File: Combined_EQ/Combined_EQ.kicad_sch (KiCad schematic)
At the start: 25 parts, among them IC2 OPA1644AIPWR

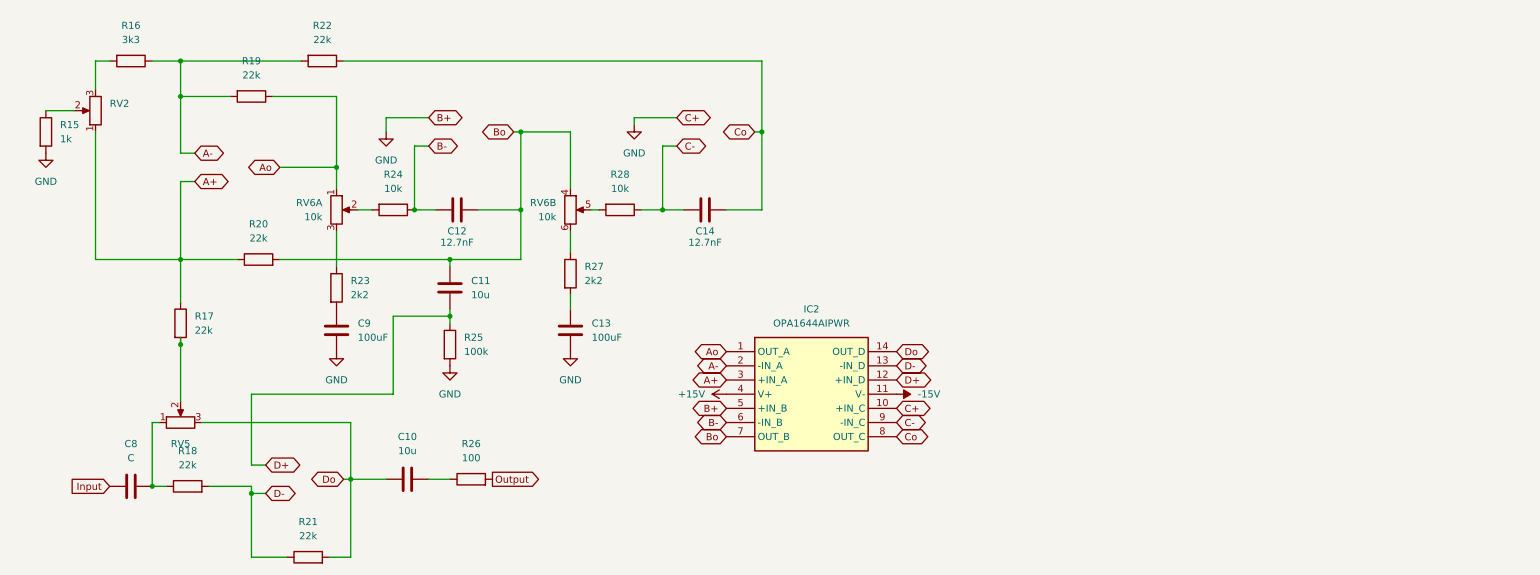
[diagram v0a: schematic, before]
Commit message: yurrrr
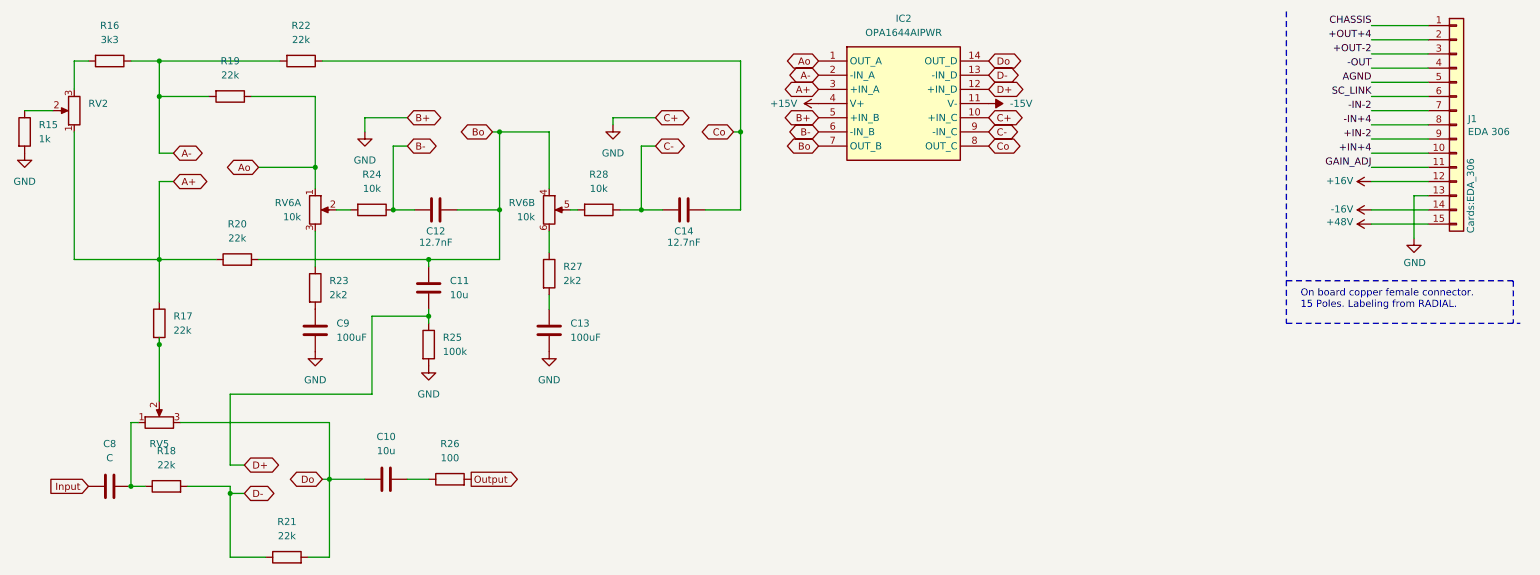
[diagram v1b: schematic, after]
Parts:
- added J1: EDA 306, Cards:EDA_306, symbol Connector_Generic:Conn_01x15
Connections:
- net GND: now also J1.13 (Pin_13)
- new net +16V: J1.12 (Pin_12)
- new net +48V: J1.15 (Pin_15)
- new net +IN+4: J1.10 (Pin_10)
- new net +IN-2: J1.9 (Pin_9)
- new net +OUT+4: J1.2 (Pin_2)
- new net +OUT-2: J1.3 (Pin_3)
- new net -16V: J1.14 (Pin_14)
- new net -IN+4: J1.8 (Pin_8)
- new net -IN-2: J1.7 (Pin_7)
- new net -OUT: J1.4 (Pin_4)
- new net AGND: J1.5 (Pin_5)
- new net CHASSIS: J1.1 (Pin_1)
- new net GAIN_ADJ: J1.11 (Pin_11)
- new net SC_LINK: J1.6 (Pin_6)
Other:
- note added: "On board copper female connector. 15 Poles. Labeling from RADIAL."
- title: High Bandpass Filter -> API Series 500 (EDA 306)
- moved on the sheet: C10, C11, C12, C13, C14, C8, C9, IC2, R15, R16, R17, R18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

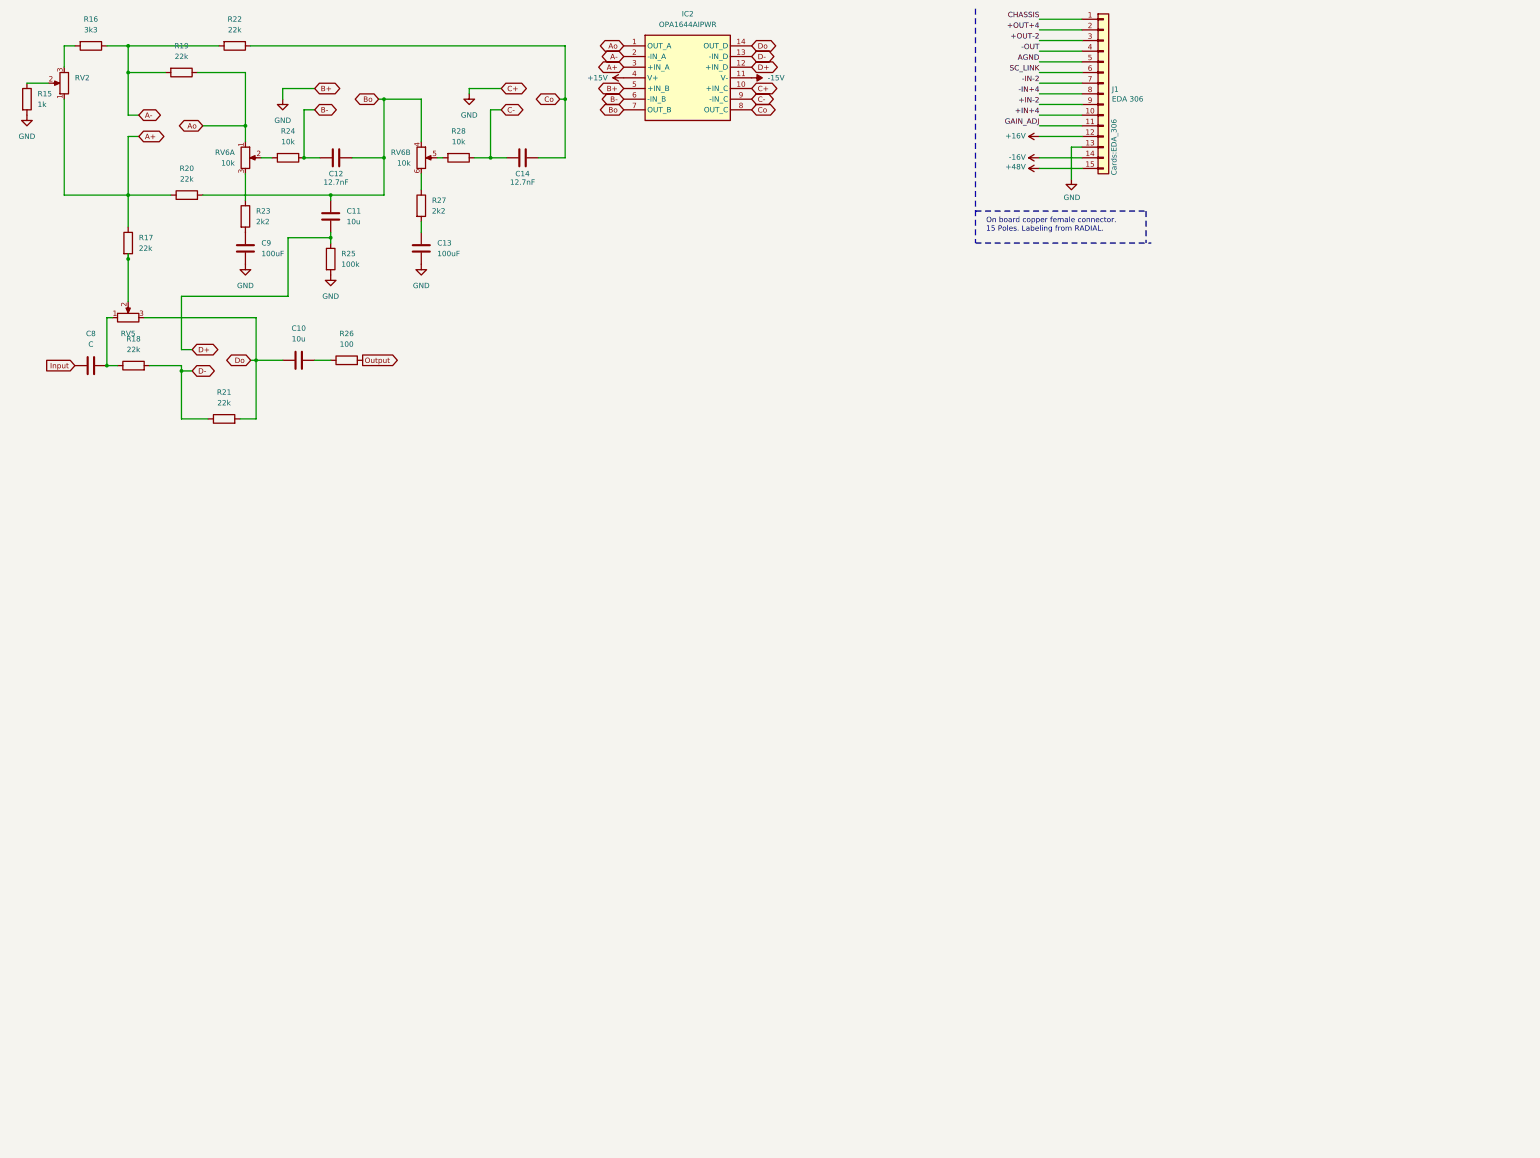
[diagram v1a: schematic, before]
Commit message: started main schematic
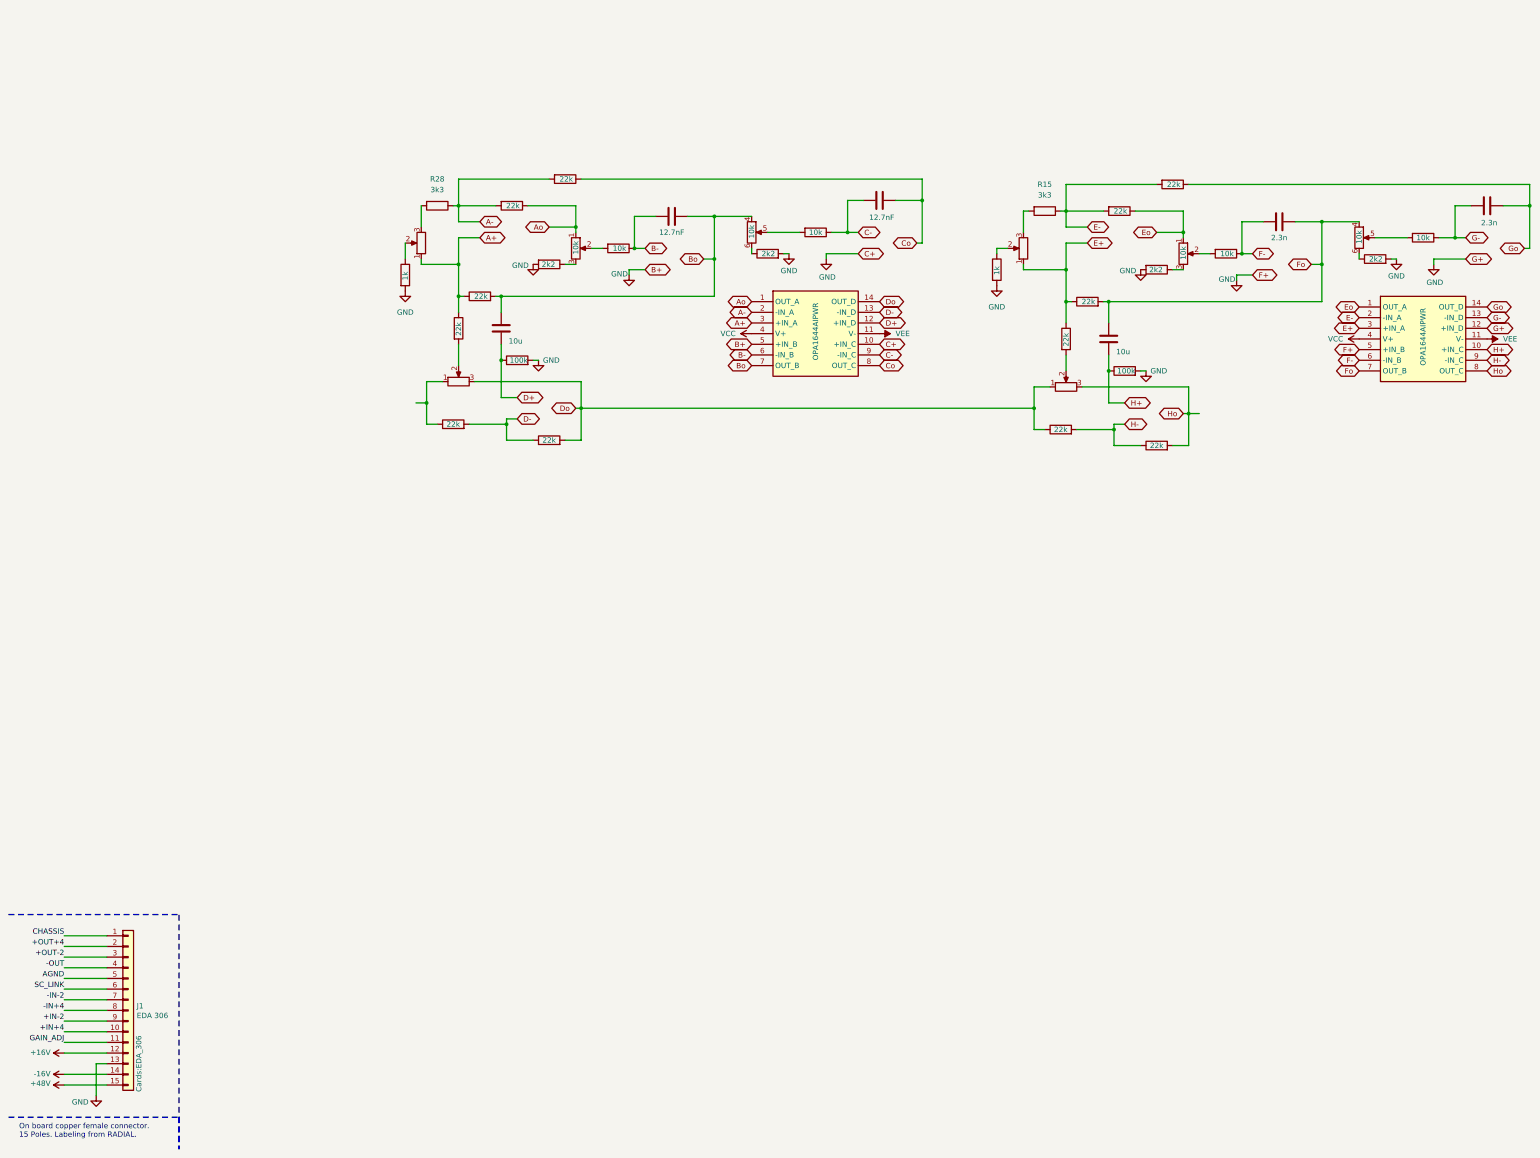
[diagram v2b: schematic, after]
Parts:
- removed C10, C11: 10u, symbol Device:C
- removed C12, C14: 12.7nF, symbol Device:C
- removed C13: 100uF, symbol Device:C
- added C2, C7: 10u, symbol Device:C
- added C3, C6: 2.3n, symbol Device:C
- added IC3: OPA1644AIPWR, SOP65P640X120-14N, symbol OPA1644AIPWR:OPA1644AIPWR
- added R14: 1k, Resistor_THT:R_Axial_DIN0207_L6.3mm_D2.5mm_P10.16mm_Horizontal, symbol Device:R
- added R29, R30, R31, R32, R35, R39: 22k, Resistor_THT:R_Axial_DIN0207_L6.3mm_D2.5mm_P10.16mm_Horizontal, symbol Device:R
- added R33: 100k, Resistor_THT:R_Axial_DIN0207_L6.3mm_D2.5mm_P10.16mm_Horizontal, symbol Device:R
- added R34, R37: 2k2, Resistor_THT:R_Axial_DIN0207_L6.3mm_D2.5mm_P10.16mm_Horizontal, symbol Device:R
- added R36, R38: 10k, Resistor_THT:R_Axial_DIN0207_L6.3mm_D2.5mm_P10.16mm_Horizontal, symbol Device:R
- added RV7, RV8: 10k, symbol Device:R_Potentiometer
- added RV9: 10k, symbol Device:R_Potentiometer_Dual_Separate
- C8: value C -> 12.7nF
- C9: value 100uF -> 12.7nF
- R15: value 1k -> 3k3
- R16: value 3k3 -> 22k
- R20: value 22k -> 100k
- R21: value 22k -> 2k2
- R23: value 2k2 -> 22k
- R25: value 100k -> 2k2
- R26: value 100 -> 10k
- R27: value 2k2 -> 1k
- R28: value 10k -> 3k3
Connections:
- net Input is gone; now on net Bo: C8.2
- net Output is gone; now on an unnamed net: R26.2
- net A+: now also IC3.3 (+IN_A), R30.1, R31.1, RV7.1; no longer IC2.3 (+IN_A), R17.1, R20.1, RV2.1
- net A-: now also R28.1, IC3.2 (-IN_A), R32.2, R35.2; no longer IC2.2 (-IN_A), R16.1, R19.2, R22.2
- net Ao: now also IC3.1 (OUT_A), R32.1, RV9.1; no longer IC2.1 (OUT_A), R19.1, RV6.1
- net B-: now also C8.1, IC3.6 (-IN_B), R36.1; no longer IC2.6 (-IN_B), R24.1
- net Bo: now also C7.2, IC3.7 (OUT_B), R31.2, RV9.4; no longer IC2.7 (OUT_B), R20.2, RV6.4
- net C-: now also C9.1, IC3.9 (-IN_C), R38.1; no longer IC2.9 (-IN_C), R28.1
- net Co: now also C9.2, IC3.8 (OUT_C), R35.1; no longer IC2.8 (OUT_C), R22.1
- net D+: now also C7.1, IC3.12 (+IN_D), R33.1; no longer IC2.12 (+IN_D), R25.1
- net D-: now also IC3.13 (-IN_D), R29.2, R39.1; no longer IC2.13 (-IN_D), R18.2, R21.1
- net Do: now also R16.1, RV5.1, IC3.14 (OUT_D), R39.2, RV8.3; no longer IC2.14 (OUT_D), R21.2, RV5.3
- net GND: now also IC2.12 (+IN_D), R20.2, R21.2, R27.2, IC3.10 (+IN_C), IC3.5 (+IN_B), R14.2, R33.2, R34.2, R37.2; no longer C9.1, IC2.10 (+IN_C), R15.2
- net at RV2.3: now also R15.2; no longer R16.2
- net at RV2.2: now also R14.1; no longer R15.1
- net at RV6.3: now also R21.1; no longer R23.1
- net E-: now reaches R23.2
- net E-: now also IC2.2 (-IN_A), R15.1, R19.2; no longer C9.2
- net G-: now reaches R26.1
- net G-: now also IC2.13 (-IN_D), C6.1
- net at RV6.5: no longer R28.2
- net at R27.1: now also RV7.2; no longer RV6.6
- net +15V renamed VCC
- net VCC: now also IC3.4 (V+)
- net -15V renamed VEE
- net VEE: now also IC3.11 (V-)
- new net: R38.2, RV9.5
- new net: R29.1, RV8.1
- new net: R30.2, RV8.2
- new net: R37.1, RV9.6
- new net: R28.2, RV7.3
- new net: R34.1, RV9.3
- new net: R25.1, RV6.6
- new net: R36.2, RV9.2
- new net E+: IC2.3 (+IN_A), R17.1, R18.1, RV2.1
- new net Eo: IC2.1 (OUT_A), R19.1, RV6.1
- new net F-: C3.1, IC2.6 (-IN_B), R24.1
- new net Fo: C2.2, C3.2, IC2.7 (OUT_B), R18.2, RV6.4
- new net Go: C6.2, IC2.14 (OUT_D), R23.1
- new net H+: C2.1, IC2.10 (+IN_C), R20.1
- new net H-: IC2.9 (-IN_C), R16.2, R22.1
- new net Ho: IC2.8 (OUT_C), R22.2, RV5.3
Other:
- moved on the sheet: J1

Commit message: worked on combined eq plus fixed a few things in gain, LPF and Bandpass
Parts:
- added C1, C5: 470p, symbol Device:C
- added C10, C4: 47u, symbol Device:C
- added C11, C12, C23: 1u, symbol Device:C
- added C13, C14, C15, C16, C17, C19, C21, C22, C30, C31: 100n, symbol Device:C
- added C18, C20, C28, C32: 100u, symbol Device:C
- added C24, C27: 20n, symbol Device:C
- added C25, C26: 270p, symbol Device:C
- added C29, C33: 220p, symbol Device:C
- added IC1: INA137PA, DIP794W53P254L959H508Q8N, symbol INA137PA:INA137PA
- added IC4, IC5: OPA1644AIPWR, OPA1644:SOP65P640X120-14N, symbol OPA1644AIPWR:OPA1644AIPWR
- added R1, R3: 47, symbol Device:R
- added R10, R41: 27K, symbol Device:R
- added R11, R43: 16K, symbol Device:R
- added R12: 5.6K, symbol Device:R
- added R13, R44: 10K, symbol Device:R
- added R2, R4, R7: 100k, symbol Device:R
- added R40, R42: 30K, symbol Device:R
- added R45, R46, R47, R48: 4.7K, symbol Device:R
- added R5, R6: 10, symbol Device:R
- added R8, R9: 6.2K, symbol Device:R
- added RV1, RV4: 100K, symbol Device:R_Potentiometer_Dual_Separate
- added RV10, RV3: 10K, symbol Device:R_Potentiometer
- IC2, IC3: footprint SOP65P640X120-14N -> OPA1644:SOP65P640X120-14N
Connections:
- net AGND is gone; now on net GND: J1.5 (Pin_5)
- net +16V: now also IC3.4 (V+), C12.2, C13.1, C19.2, C20.2, IC1.7 (V+), R6.1; no longer J1.12 (Pin_12)
- net +IN+4: now also R3.1
- net -16V: now also IC2.11 (V-), IC2.4 (V+), IC3.11 (V-), C11.2, C14.1, C15.1, C16.1, C17.1, C18.1, C21.1, C22.1, C30.1, C31.1, IC1.4 (V-), IC4.11 (V-), IC4.4 (V+), IC5.11 (V-), IC5.4 (V+), R5.1; no longer J1.14 (Pin_14)
- net -IN+4: now also R1.1
- net CHASSIS: now also C1.2, C5.2
- net GND: now also C11.1, C12.1, C13.2, C14.2, C15.2, C16.2, C17.2, C18.2, C19.1, C20.1, C21.2, C22.2, C27.1, C30.2, C31.2, IC1.1 (REF), R10.2, R13.2, R2.1, R4.1, R41.2, R7.1, RV4.3
- net Ho: now also C23.1
- net VCC: now also J1.12 (Pin_12), R6.2; no longer IC2.4 (V+), IC3.4 (V+)
- net VEE: now also J1.14 (Pin_14), R5.2; no longer IC2.11 (V-), IC3.11 (V-)
- net I-: now reaches R29.1, RV8.1
- net I-: now also IC4.1 (OUT_A), IC4.2 (-IN_A)
- net +48V: no longer names the net of J1.15 (Pin_15)
- net +IN-2: no longer names the net of J1.9 (Pin_9)
- net +OUT-2: no longer names the net of J1.3 (Pin_3)
- net -IN-2: no longer names the net of J1.7 (Pin_7)
- net GAIN_ADJ: no longer names the net of J1.11 (Pin_11)
- new net: C10.1, C5.1, R3.2
- new net: C10.2, IC1.3 (+IN), R4.2
- new net: C28.1, R45.1
- new net: R8.2, RV1.1, RV1.2
- new net: C4.2, IC1.2 (-IN), R2.2
- new net: C24.2, R9.1, RV1.3
- new net: R9.2, RV1.4, RV1.5
- new net: R48.1, RV10.1
- new net: R47.2, RV10.3
- new net: C1.1, C4.1, R1.2
- new net: C25.2, C26.1, R40.1
- new net: C25.1, R12.1, R13.1
- new net: R42.2, RV4.1, RV4.2
- new net: R45.2, RV3.3
- new net: C32.1, R47.1
- new net: R46.1, RV3.1
- new net: R40.2, RV4.4, RV4.5
- new net I+: IC1.5 (SENSE), IC1.6 (OUTPUT), IC4.3 (+IN_A)
- new net J+: C23.2, IC4.5 (+IN_B), R7.2
- new net J-: IC4.6 (-IN_B), IC4.7 (OUT_B), R12.2, R44.2, R8.1
- new net K+: C27.2, IC4.12 (+IN_D), RV1.6
- new net K-: IC4.13 (-IN_D), R10.1, R11.1
- new net Ko: C24.1, C28.2, IC4.14 (OUT_D), R11.2
- new net L+: C26.2, IC4.10 (+IN_C), R42.1
- new net L-: IC4.9 (-IN_C), R41.1, R43.1
- new net Lo: C32.2, IC4.8 (OUT_C), R43.2, RV4.6
- new net M-: C29.1, C33.1, RV10.2, RV3.2
- new net Mo: C29.2, C33.2, R46.2, R48.2
- no-connect marks 0 -> 5
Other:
- note added: "500 SERIES CONNECTOR"
- note added: "BALANCED INPUT RECIEVER"
- note added: "BUFFER"
- note added: "HIGH BANDPASS FILTER"
- note added: "HIGH PASS FILTER"
- note added: "LOW BANDPASS FILTER"
- note added: "LOW PASS FILTER"
- note added: "RAIL FILTERING"
- note added: "VARIABLE GAIN"
- note removed: "On board copper female connector. 15 Poles. Labeling from RADIAL."
- moved on the sheet: R15, R28
